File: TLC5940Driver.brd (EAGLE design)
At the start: 72.9 x 52.4 mm, 85 parts, among them IC1 ATMEGA88PA, IC2 SPX3819, IC3 TLC5940, IC4 TLC5940, IC5 TLC5940

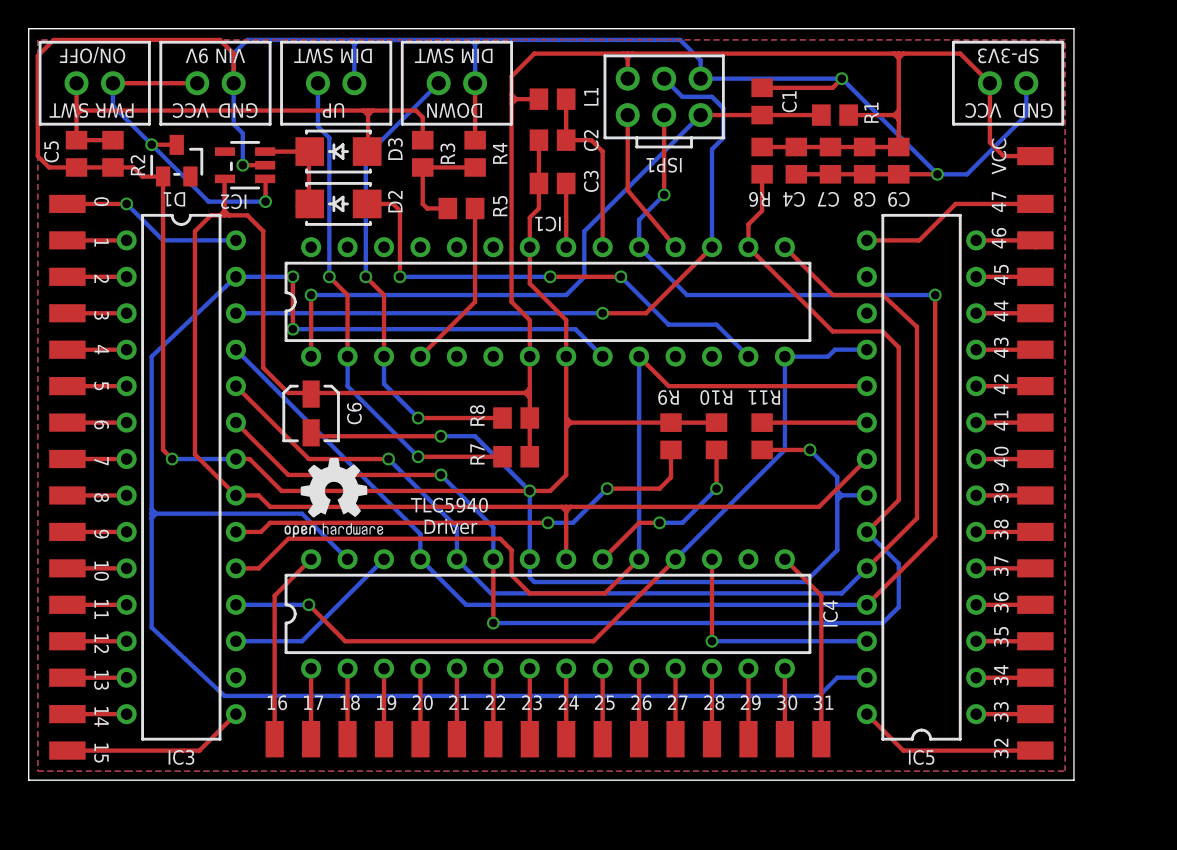
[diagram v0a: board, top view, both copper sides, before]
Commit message: Update TLC5940Driver.brd
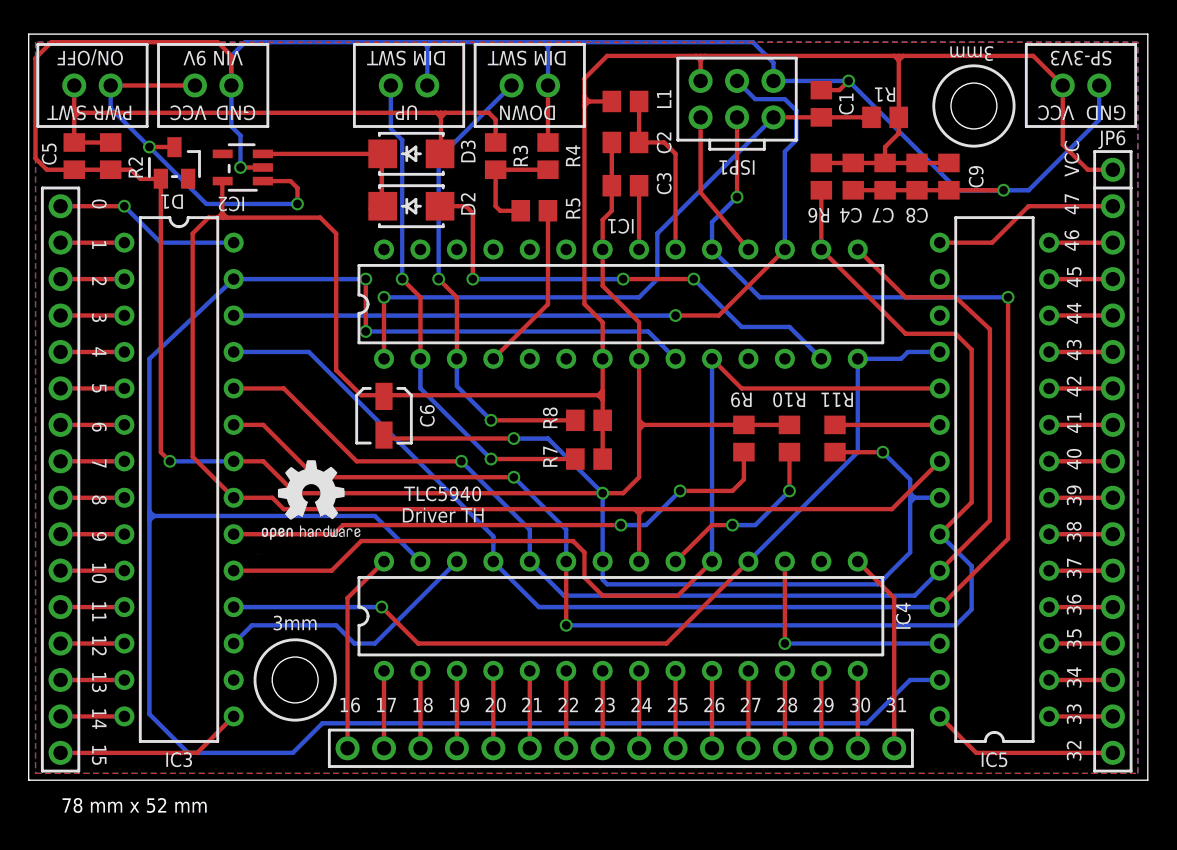
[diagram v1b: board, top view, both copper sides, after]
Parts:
- removed PAD1, PAD10, PAD11, PAD12, PAD13, PAD14, PAD15, PAD16, PAD17, PAD18, PAD19, PAD2, PAD20, PAD21, PAD22, PAD23, PAD24, PAD25, PAD26, PAD27, PAD28, PAD29, PAD3, PAD30, PAD31, PAD32, PAD33, PAD34, PAD35, PAD36, PAD37, PAD38, PAD39, PAD4, PAD40, PAD41, PAD42, PAD43, PAD44, PAD45, PAD46, PAD47, PAD48, PAD49, PAD5, PAD6, PAD7, PAD8, PAD9: (no value), wirepad:SMD1,27-2,54
- added JP3, JP4, JP5: (no value), dn-electronics:P-1X16
- added JP6: (no value), dn-electronics:P-1X01
- moved IC5 5.08 mm to (67.3, 21.0)
- moved ISP1 5.08 mm to (49.4, 47.5)
- moved R7 5.08 mm to (39.1, 22.4)
- moved R8 5.08 mm to (39.1, 25.1)
- moved C6 5.08 mm to (24.8, 25.4)
- moved D2 5.08 mm to (26.7, 40.0)
- moved D3 5.08 mm to (26.7, 43.7)
- moved R3 5.08 mm to (32.5, 43.5)
- moved R4 5.08 mm to (36.2, 43.5)
- moved SW3 5.08 mm to (26.5, 48.4)
- moved C2 5.08 mm to (41.6, 44.5)
- moved C3 5.08 mm to (41.6, 41.4)
- moved IC1 5.08 mm to (41.3, 33.2)
- moved IC4 5.08 mm to (41.3, 11.4)
- moved JP2 5.08 mm to (73.3, 48.4)
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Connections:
- net N$10: now also JP3.7; no longer PAD8.1
- net N$11: now also JP3.8; no longer PAD9.1
- net N$12: now also JP3.9; no longer PAD10.1
- net N$13: now also JP3.10; no longer PAD11.1
- net N$14: now also JP3.11; no longer PAD12.1
- net N$15: now also JP3.12; no longer PAD13.1
- net N$16: now also JP3.13; no longer PAD14.1
- net N$17: now also JP3.14; no longer PAD15.1
- net N$18: now also JP3.15; no longer PAD16.1
- net N$19: now also JP3.16; no longer PAD17.1
- net N$20: now also JP4.1; no longer PAD18.1
- net N$21: now also JP4.2; no longer PAD19.1
- net N$22: now also JP4.3; no longer PAD20.1
- net N$23: now also JP4.4; no longer PAD21.1
- net N$24: now also JP4.5; no longer PAD22.1
- net N$25: now also JP4.6; no longer PAD23.1
- net N$26: now also JP4.7; no longer PAD24.1
- net N$27: now also JP4.8; no longer PAD25.1
- net N$28: now also JP4.9; no longer PAD26.1
- net N$29: now also JP4.10; no longer PAD27.1
- net N$3: now also JP3.1; no longer PAD2.1
- net N$30: now also JP4.11; no longer PAD28.1
- net N$31: now also JP4.12; no longer PAD29.1
- net N$32: now also JP4.13; no longer PAD30.1
- net N$33: now also JP4.14; no longer PAD31.1
- net N$34: now also JP4.15; no longer PAD32.1
- net N$35: now also JP4.16; no longer PAD33.1
- net N$36: now also JP5.1; no longer PAD34.1
- net N$37: now also JP5.2; no longer PAD35.1
- net N$38: now also JP5.3; no longer PAD36.1
- net N$39: now also JP5.4; no longer PAD37.1
- net N$40: now also JP5.5; no longer PAD38.1
- net N$41: now also JP5.6; no longer PAD39.1
- net N$42: now also JP5.7; no longer PAD40.1
- net N$43: now also JP5.8; no longer PAD41.1
- net N$44: now also JP5.9; no longer PAD42.1
- net N$45: now also JP5.10; no longer PAD43.1
- net N$46: now also JP5.11; no longer PAD44.1
- net N$47: now also JP5.12; no longer PAD45.1
- net N$48: now also JP5.13; no longer PAD46.1
- net N$49: now also JP5.14; no longer PAD47.1
- net N$5: now also JP3.2; no longer PAD3.1
- net N$50: now also JP5.15; no longer PAD48.1
- net N$51: now also JP5.16; no longer PAD49.1
- net N$6: now also JP3.3; no longer PAD4.1
- net N$7: now also JP3.4; no longer PAD5.1
- net N$8: now also JP3.5; no longer PAD6.1
- net N$9: now also JP3.6; no longer PAD7.1
- net VCC: now also JP6.1; no longer PAD1.1
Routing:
- net N$70: track 125.1 -> 147.5 mm
- net GND: track 278.8 -> 287.1 mm
- net VCC: track 205.8 -> 213.2 mm
- net N$65: track 12.7 -> 19.0 mm
- net N$2: track 38.3 -> 43.9 mm
- net N$4: track 8.09 -> 13.3 mm
- net N$67: track 81.7 -> 87.0 mm
- net N$74: track 33.8 -> 39.0 mm
- net N$69: track 63.4 -> 68.6 mm
- net N$68: track 57.3 -> 62.5 mm
- net N$60: track 50.1 -> 55.3 mm
- net N$58: track 107.9 -> 113.1 mm
- net N$1: track 24.2 -> 28.7 mm
- net N$52: track 95.1 -> 99.0 mm
- net N$55: track 46.9 -> 45.3 mm
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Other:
- board size 72.9 x 52.4 mm -> 78 x 52 mm
- board text added: "3mm"
- board text added: "78 mm x 52 mm"
- board text added: "TLC5940 Driver TH"
- board text removed: "TLC5940 Driver"
